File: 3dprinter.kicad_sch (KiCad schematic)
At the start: 28 parts, among them J1 6P IDC CONNECTOR, J2 USB_B_Micro, J3 Conn_01x02, SW1 6x6 SMD, U1 ATmega2560-16A, Y1 16MHz

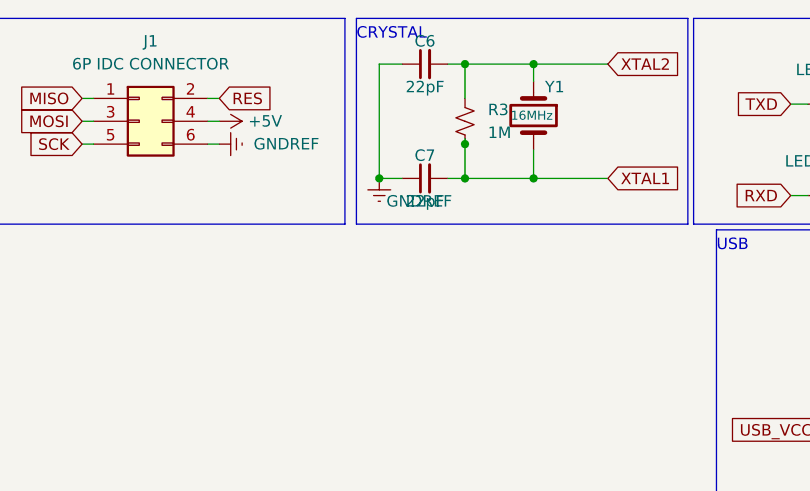
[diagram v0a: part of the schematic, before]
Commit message: comm
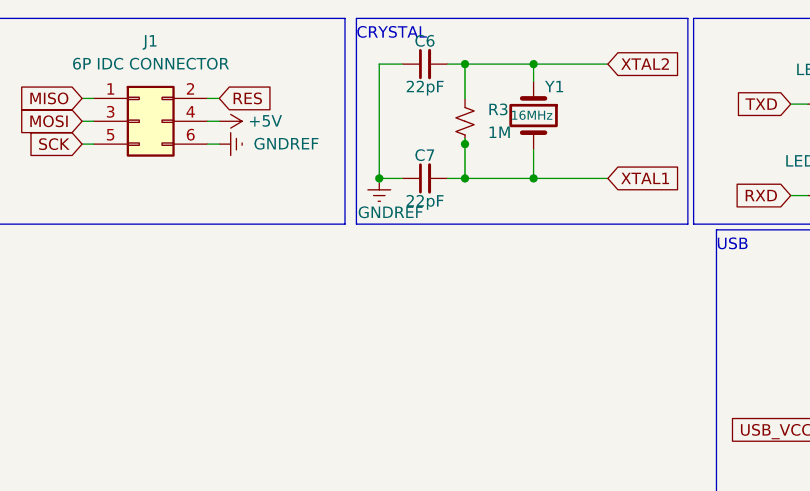
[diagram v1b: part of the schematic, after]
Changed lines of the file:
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@@
       (effects (font (size 1.27 1.27)) hide)
     )
-    (property "Value" "GNDREF" (id 1) (at 163.195 33.02 0))
+    (property "Value" "GNDREF" (id 1) (at 160.02 34.29 0))
     (property "Footprint" "" (id 2) (at 158.75 30.48 0)
       (effects (font (size 1.27 1.27)) hide)
